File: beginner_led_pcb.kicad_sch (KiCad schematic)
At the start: 8 parts, among them J1 Conn_01x03_Pin

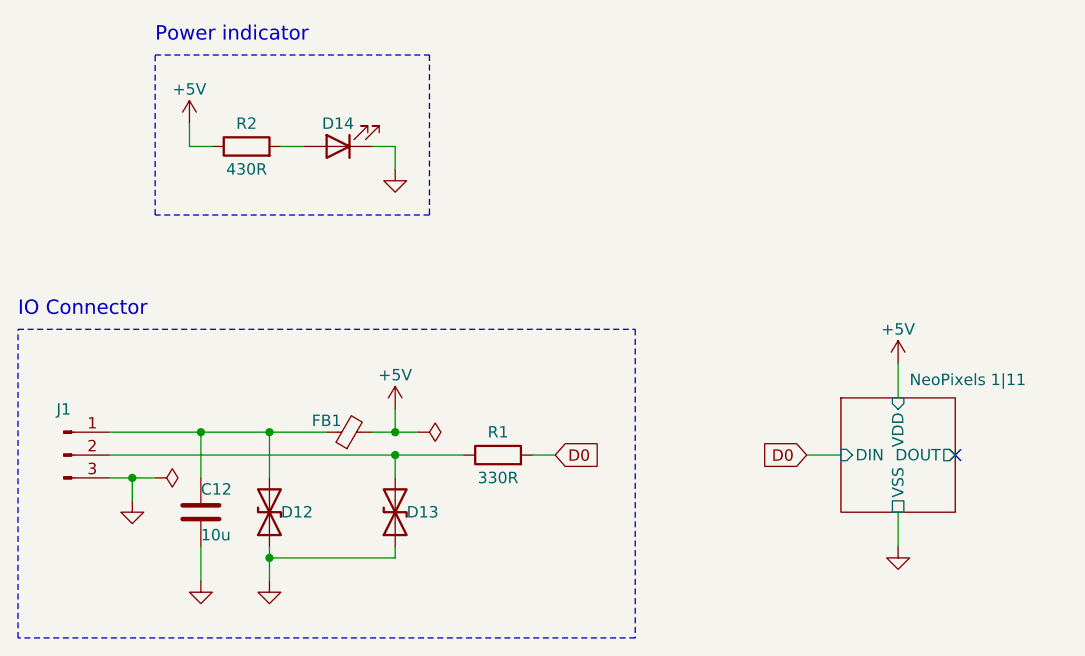
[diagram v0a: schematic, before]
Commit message: new components
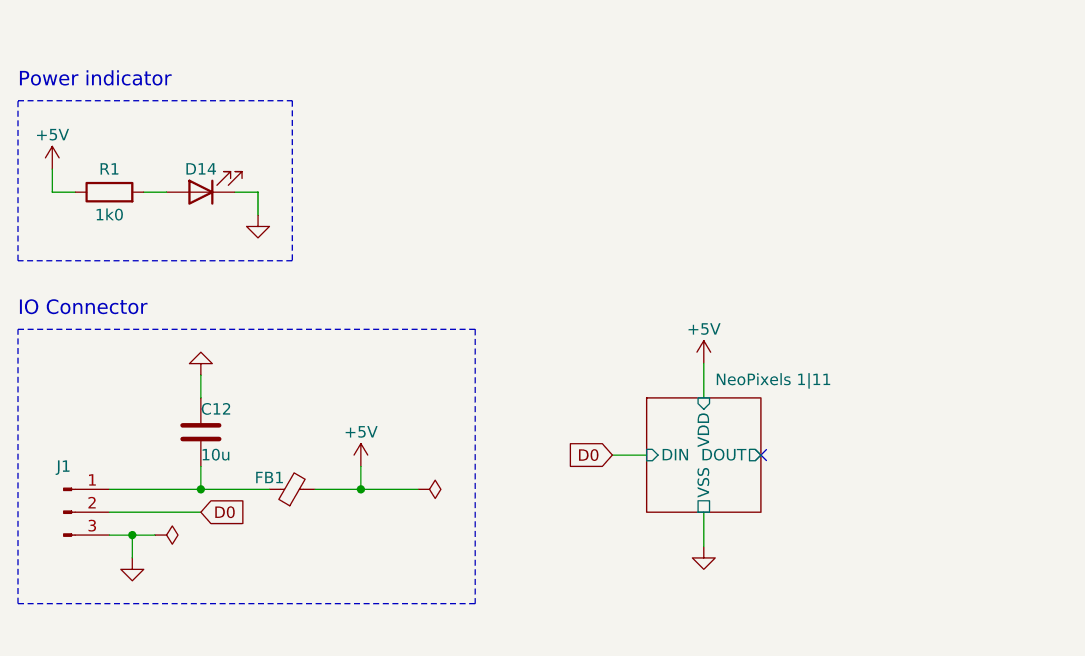
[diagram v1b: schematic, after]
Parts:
- removed D12, D13: D_TVS, Diode_SMD:D_SOD-323, symbol Device:D_TVS
- removed R1: 330R, Resistor_SMD:R_0603_1608Metric, symbol Device:R
- C12: JLCPCB Part # (none) -> C2169262
- FB1: footprint Inductor_SMD:L_0603_1608Metric -> Inductor_SMD:L_0805_2012Metric; JLCPCB Part # (none) -> C111240
- J1: JLCPCB Part # (none) -> C2883841
- R1: renamed from R2; value 430R -> 1k0; JLCPCB Part # (none) -> C21190
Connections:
- net D0: now also J1.2 (Pin_2)
- net GND: now also C12.1; no longer C12.2
- net at FB1.1, J1.1 (Pin_1): now also C12.2; no longer C12.1
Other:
- moved on the sheet: C12, D14, FB1, J1, R1
